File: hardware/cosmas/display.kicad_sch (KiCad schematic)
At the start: 1 part, among them J2 I2C_LCD_SCREEN

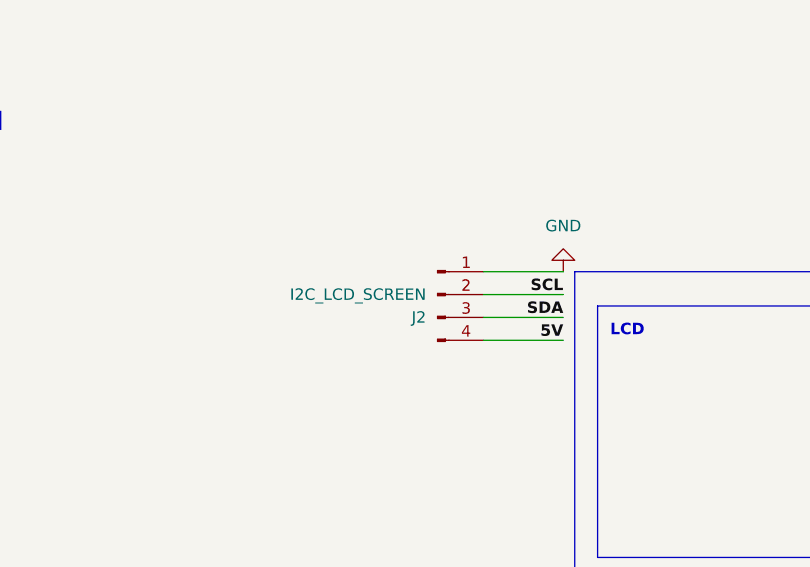
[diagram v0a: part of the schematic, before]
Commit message: adds OBC PCB
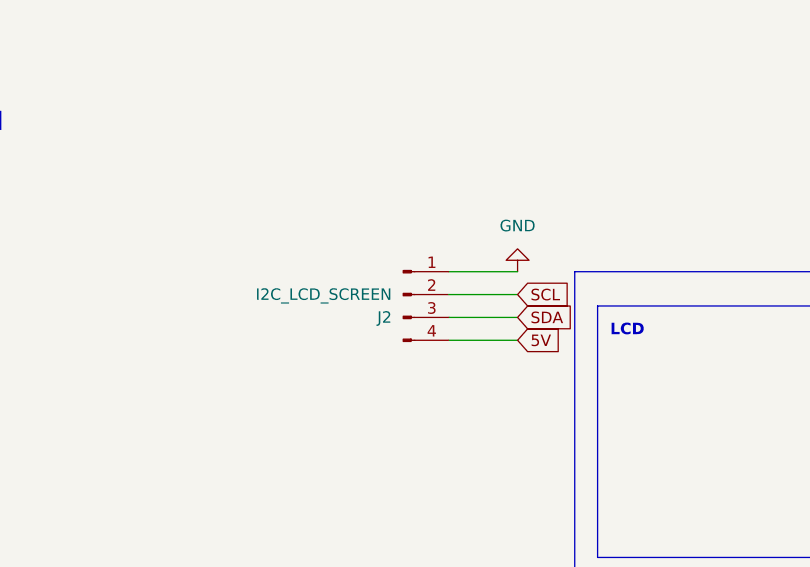
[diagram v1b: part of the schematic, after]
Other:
- moved on the sheet: J2
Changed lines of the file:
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@@
 	(wire
 		(pts
-			(xy 129.54 87.63) (xy 120.65 87.63)
-		)
-		(stroke
-			(width 0)
-			(type default)
-		)
-	)
-	(wire
-		(pts
-			(xy 129.54 85.09) (xy 120.65 85.09)
-		)
-		(stroke
-			(width 0)
-			(type default)
-		)
-	)
-	(wire
-		(pts
-			(xy 129.54 90.17) (xy 120.65 90.17)
-		)
-		(stroke
-			(width 0)
-			(type default)
-		)
-	)
-	(wire
-		(pts
-			(xy 129.54 92.71) (xy 120.65 92.71)
+			(xy 124.46 87.63) (xy 116.84 87.63)
+		)
+		(stroke
+			(width 0)
+			(type default)
+		)
+	)
+	(wire
+		(pts
+			(xy 124.46 85.09) (xy 116.84 85.09)
+		)
+		(stroke
+			(width 0)
+			(type default)
+		)
+	)
+	(wire
+		(pts
+			(xy 124.46 90.17) (xy 116.84 90.17)
+		)
+		(stroke
+			(width 0)
+			(type default)
+		)
+	)
+	(wire
+		(pts
+			(xy 124.46 92.71) (xy 116.84 92.71)
 		)
 		(stroke
@@
 		)
 	)
-	(label "SCL"
-		(at 129.54 87.63 180)
-		(fields_autoplaced yes)
-		(effects
-			(font
-				(size 1.27 1.27)
-				(bold yes)
-			)
-			(justify right bottom)
-		)
-	)
-	(label "SDA"
-		(at 129.54 90.17 180)
-		(fields_autoplaced yes)
-		(effects
-			(font
-				(size 1.27 1.27)
-				(bold yes)
-			)
-			(justify right bottom)
-		)
-	)
-	(label "5V"
-		(at 129.54 92.71 180)
-		(fields_autoplaced yes)
-		(effects
-			(font
-				(size 1.27 1.27)
-				(bold yes)
-			)
-			(justify right bottom)
+	(global_label "5V"
+		(shape input)
+		(at 124.46 92.71 0)
+		(fields_autoplaced yes)
+		(effects
+			(font
+				(size 1.27 1.27)
+			)
+			(justify left)
+		)
+		(property "Intersheetrefs" "${INTERSHEET_REFS}"
+			(at 129.7433 92.71 0)
+			(effects
+				(font
+					(size 1.27 1.27)
+				)
+				(justify left)
+				(hide yes)
+			)
+		)
+	)
+	(global_label "SDA"
+		(shape input)
+		(at 124.46 90.17 0)
+		(fields_autoplaced yes)
+		(effects
+			(font
+				(size 1.27 1.27)
+			)
+			(justify left)
+		)
+		(property "Intersheetrefs" "${INTERSHEET_REFS}"
+			(at 131.0133 90.17 0)
+			(effects
+				(font
+					(size 1.27 1.27)
+				)
+				(justify left)
+				(hide yes)
+			)
+		)
+	)
+	(global_label "SCL"
+		(shape input)
+		(at 124.46 87.63 0)
+		(fields_autoplaced yes)
+		(effects
+			(font
+				(size 1.27 1.27)
+			)
+			(justify left)
+		)
+		(property "Intersheetrefs" "${INTERSHEET_REFS}"
+			(at 130.9528 87.63 0)
+			(effects
+				(font
+					(size 1.27 1.27)
+				)
+				(justify left)
+				(hide yes)
+			)
 		)
 	)
 	(symbol
 		(lib_id "Connector:Conn_01x04_Pin")
-		(at 115.57 87.63 0)
+		(at 111.76 87.63 0)
 		(unit 1)
 		(exclude_from_sim no)
@@
 		(fields_autoplaced yes)
 		(property "Reference" "J2"
-			(at 114.3 90.1701 0)
+			(at 110.49 90.1701 0)
 			(effects
 				(font
@@
 		)
 		(property "Value" "I2C_LCD_SCREEN"
-			(at 114.3 87.6301 0)
+			(at 110.49 87.6301 0)
 			(effects
 				(font
@@
 		)
 		(property "Footprint" "Connector_PinHeader_2.54mm:PinHeader_1x04_P2.54mm_Vertical"
-			(at 115.57 87.63 0)
+			(at 111.76 87.63 0)
 			(effects
 				(font
@@
 		)
 		(property "Datasheet" "~"
-			(at 115.57 87.63 0)
+			(at 111.76 87.63 0)
 			(effects
 				(font
@@
 		)
 		(property "Description" "Generic connector, single row, 01x04, script generated"
-			(at 115.57 87.63 0)
+			(at 111.76 87.63 0)
 			(effects
 				(font
@@
 	(symbol
 		(lib_id "power:GND")
-		(at 129.54 85.09 180)
+		(at 124.46 85.09 180)
 		(unit 1)
 		(exclude_from_sim no)
@@
 		(fields_autoplaced yes)
 		(property "Reference" "#PWR014"
-			(at 129.54 78.74 0)
+			(at 124.46 78.74 0)
 			(effects
 				(font
@@
 		)
 		(property "Value" "GND"
-			(at 129.54 80.01 0)
+			(at 124.46 80.01 0)
 			(effects
 				(font
@@
 		)
 		(property "Footprint" ""
-			(at 129.54 85.09 0)
+			(at 124.46 85.09 0)
 			(effects
 				(font
@@
 		)
 		(property "Datasheet" ""
-			(at 129.54 85.09 0)
+			(at 124.46 85.09 0)
 			(effects
 				(font
@@
 		)
 		(property "Description" "Power symbol creates a global label with name \"GND\" , ground"
-			(at 129.54 85.09 0)
-			(effects
-				(font
+			(at 124.46 85.09 0)
+			(effects
+				(font
